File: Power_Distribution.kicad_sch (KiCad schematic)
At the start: 23 parts, among them IC1 LP5912-3.3DRVR, J7 CarPowerConnector, Q1 PBSS4330X,135, Q2 SI7149ADP-T1-GE3

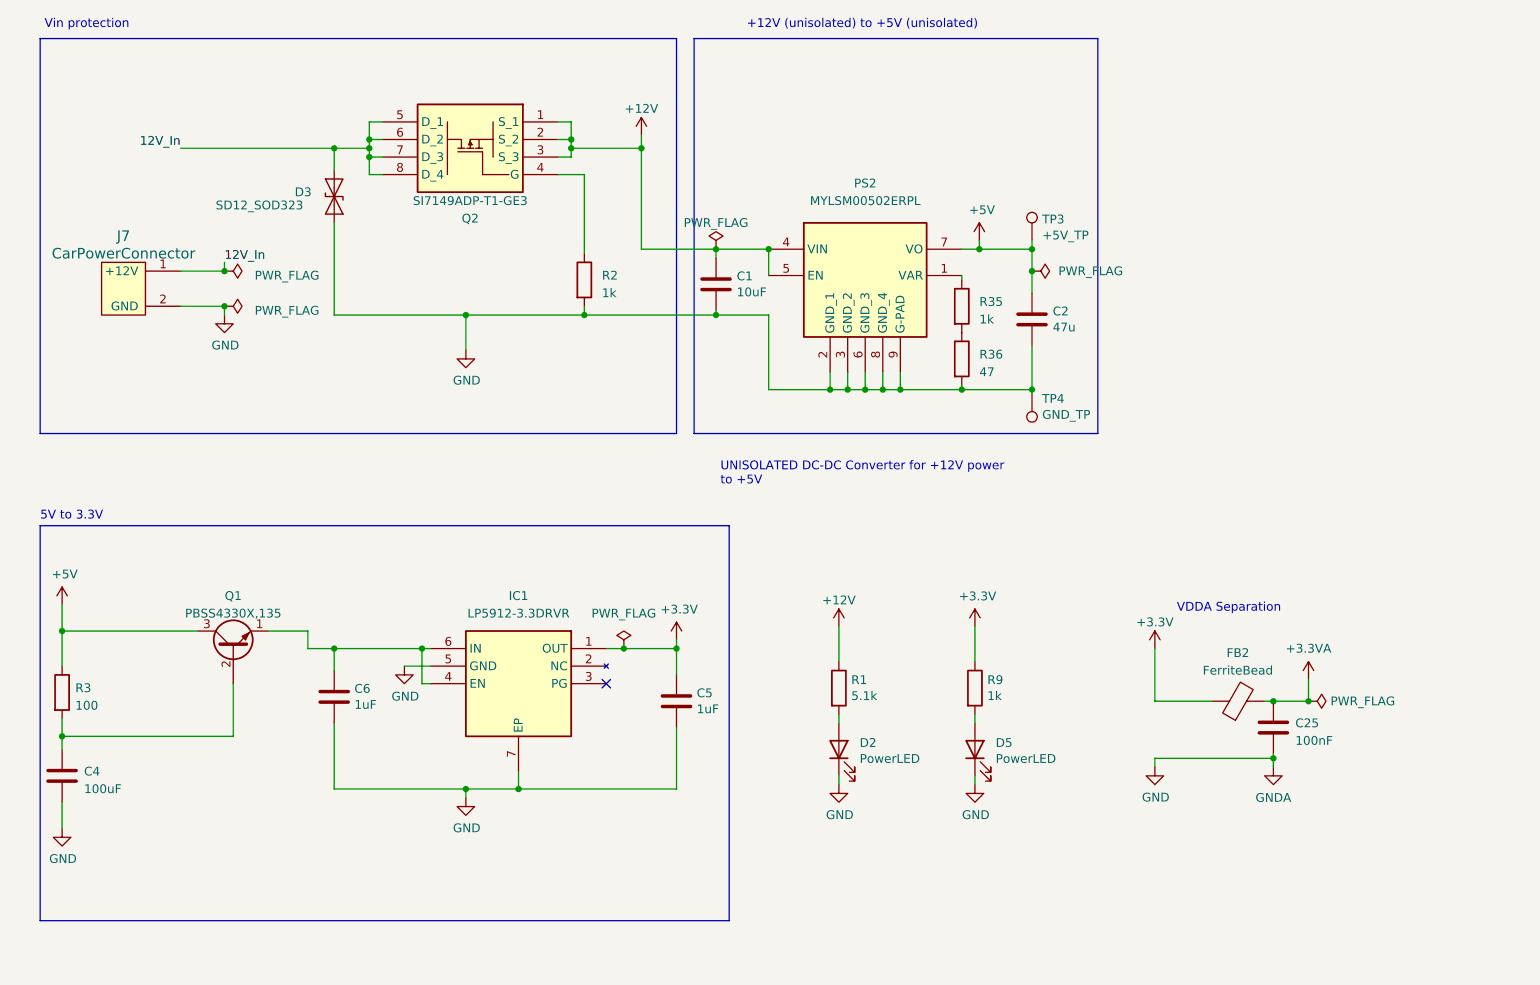
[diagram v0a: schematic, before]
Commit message: 👹
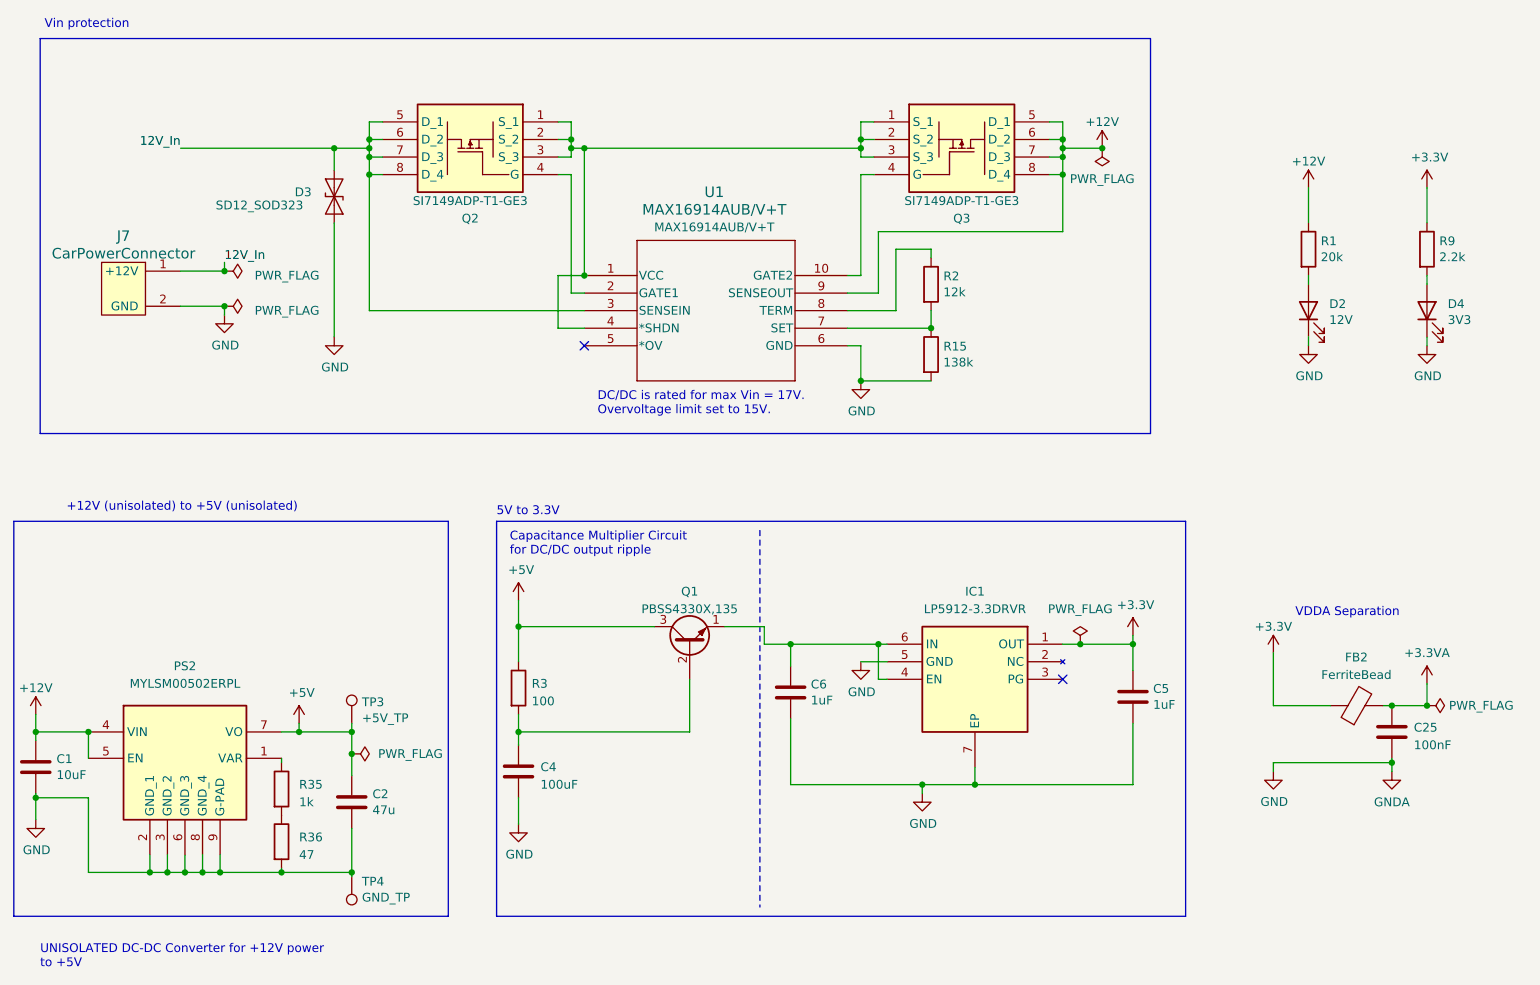
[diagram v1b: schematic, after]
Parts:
- removed D5: PowerLED, LED_SMD:LED_0805_2012Metric, symbol Device:LED
- added D4: 3V3, LED_SMD:LED_0805_2012Metric, symbol Device:LED
- added Q3: SI7149ADP-T1-GE3, UTSVT_ICs:POWERPAKSO-8, symbol utsvt-chips:SI7149ADP-T1-GE3
- added R15: 138k, Resistor_SMD:R_0805_2012Metric, symbol Device:R
- added U1: MAX16914AUB/V+T, UTSVT_ICs:21-0061L_MXM, symbol utsvt-chips:MAX16914AUB_V+T
- D2: value PowerLED -> 12V
- IC1: footprint SON65P200X200X80-7N -> UTSVT_Power:SON65P200X200X80-7N
- Q1: footprint Package_TO_SOT_THT:TO-39-3 -> Package_TO_SOT_SMD:SOT-89-3
- Q2: footprint POWERPAKSO-8 -> UTSVT_ICs:POWERPAKSO-8
- R1: value 5.1k -> 20k; Mouser Part Number 71-CRCW0805-21.5K-E3 -> Inventory; P/N CRCW080521K5FKEA -> Inventory
- R2: value 1k -> 12k; Mouser Part Number 71-CRCW08051K00FKEAC -> (none); P/N CRCW08051K00FKEAC -> (none)
- R9: value 1k -> 2.2k; Mouser Part Number 71-CRCW0805-21.5K-E3 -> Inventory; P/N CRCW080521K5FKEA -> Inventory
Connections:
- net +12V: now also Q3.5 (D_1), Q3.6 (D_2), Q3.7 (D_3), Q3.8 (D_4), U1.9 (SENSEOUT); no longer Q2.1 (S_1), Q2.2 (S_2), Q2.3 (S_3)
- net 12V_In: now also U1.3 (SENSEIN)
- net GND: now also D4.1 (K), R15.2, U1.6 (GND); no longer R2.2
- net at Q2.4 (G): now also U1.2 (GATE1); no longer R2.1
- net at R9.2: now also D4.2 (A)
- new net: Q2.1 (S_1), Q2.2 (S_2), Q2.3 (S_3), Q3.1 (S_1), Q3.2 (S_2), Q3.3 (S_3), U1.1 (VCC), U1.4 (*SHDN)
- new net: Q3.4 (G), U1.10 (GATE2)
- new net: R15.1, R2.2, U1.7 (SET)
- new net: R2.1, U1.8 (TERM)
- no-connect marks 1 -> 2
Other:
- note added: "Capacitance Multiplier Circuit for DC/DC output ripple"
- note added: "DC/DC is rated for max Vin = 17V. Overvoltage limit set to 15V."
- moved on the sheet: C1, C2, C25, C4, C5, C6, FB2, IC1, PS2, Q1, R3, R35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
